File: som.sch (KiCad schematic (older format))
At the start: 22 parts, among them J7 MC-HVT1-S04-G, M1 SA800U-WF-mechanical_model, U10 SA800U-WF

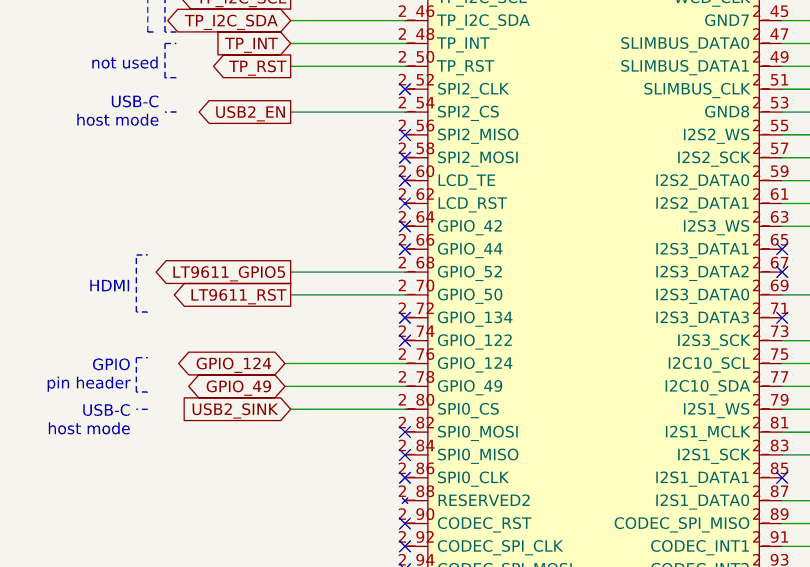
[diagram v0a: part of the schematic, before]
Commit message: Continue layout
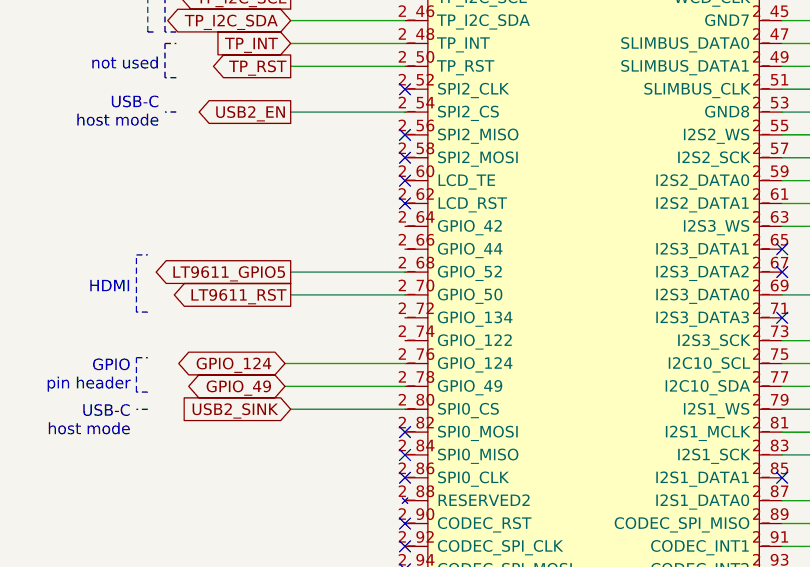
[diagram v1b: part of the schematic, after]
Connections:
- no-connect marks 58 -> 54
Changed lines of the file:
@@
 NoConn ~ 8100 4400
 NoConn ~ 8100 4500
-NoConn ~ 8100 4600
-NoConn ~ 8100 4700
-NoConn ~ 8100 5000
-NoConn ~ 8100 5100
 Wire Wire Line
 	4150 8925 4525 8925
